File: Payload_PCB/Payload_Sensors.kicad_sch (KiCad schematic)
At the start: 8 parts

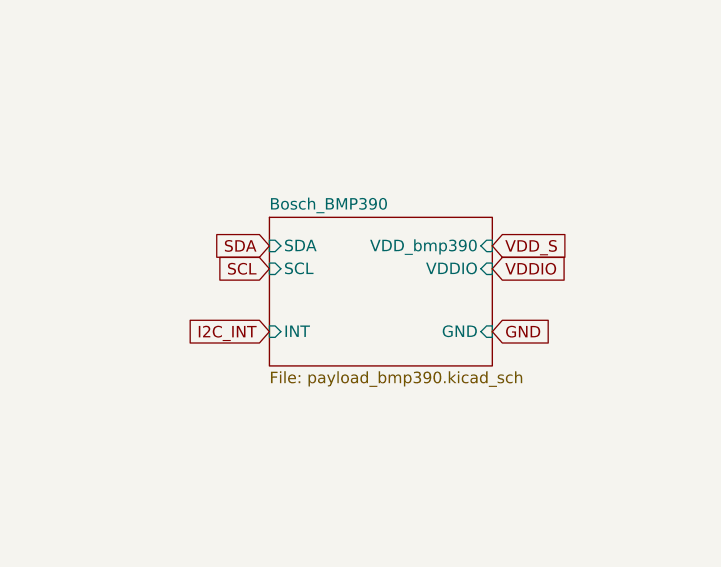
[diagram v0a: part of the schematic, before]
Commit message: some new parts
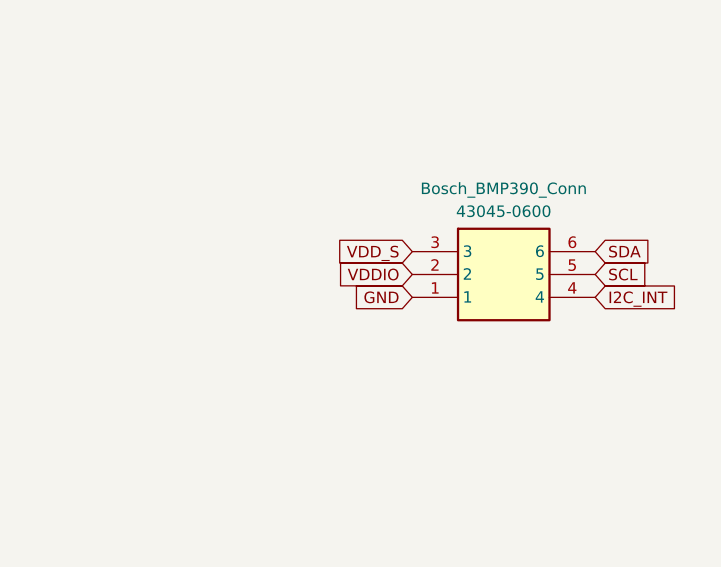
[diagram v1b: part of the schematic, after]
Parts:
- added Bosch_BMP390_Conn: 43045-0600, footprints:43045-06_00,01,02,10_, symbol 43045-0600:43045-0600
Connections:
- net GND: now also Bosch_BMP390_Conn.1
- net I2C_INT: now also Bosch_BMP390_Conn.4
- net SCL: now also Bosch_BMP390_Conn.5
- net SDA: now also Bosch_BMP390_Conn.6
- net VDDIO: now also Bosch_BMP390_Conn.2
- net VDD_S: now also Bosch_BMP390_Conn.3
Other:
- removed sheet Bosch_BMP390
- company: (none) -> SpaceTeam Aachen
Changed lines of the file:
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@@
   (title_block
     (title "Sensor Modules")
+    (company "SpaceTeam Aachen")
   )
   (junction (at 74.295 57.785) (diameter 0) (color 0 0 0 0)
@@
     )
   )
+  (global_label "SCL" (shape input) (at 166.37 210.185 0) (fields_autoplaced)
+    (effects (font (size 1.27 1.27)) (justify left))
+    (property "Intersheetrefs" "${INTERSHEET_REFS}" (at 172.8628 210.185 0)
+      (effects (font (size 1.27 1.27)) (justify left) hide)
+    )
+  )
   (global_label "GND" (shape input) (at 131.445 162.56 0) (fields_autoplaced)
     (effects (font (size 1.27 1.27)) (justify left))
@@
     )
   )
+  (global_label "SDA" (shape input) (at 166.37 207.645 0) (fields_autoplaced)
+    (effects (font (size 1.27 1.27)) (justify left))
+    (property "Intersheetrefs" "${INTERSHEET_REFS}" (at 172.9233 207.645 0)
+      (effects (font (size 1.27 1.27)) (justify left) hide)
+    )
+  )
   (global_label "VDD_TC" (shape input) (at 83.82 43.815 180) (fields_autoplaced)
     (effects (font (size 1.27 1.27)) (justify right))
@@
     )
   )
+  (global_label "GND" (shape input) (at 146.05 212.725 180) (fields_autoplaced)
+    (effects (font (size 1.27 1.27)) (justify right))
+    (property "Intersheetrefs" "${INTERSHEET_REFS}" (at 139.1943 212.725 0)
+      (effects (font (size 1.27 1.27)) (justify right) hide)
+    )
+  )
   (global_label "VDD_TC" (shape input) (at 106.68 151.765 180) (fields_autoplaced)
     (effects (font (size 1.27 1.27)) (justify right))
@@
     )
   )
-  (global_label "VDDIO" (shape input) (at 154.94 209.55 0) (fields_autoplaced)
-    (effects (font (size 1.27 1.27)) (justify left))
-    (property "Intersheetrefs" "${INTERSHEET_REFS}" (at 163.4891 209.55 0)
-      (effects (font (size 1.27 1.27)) (justify left) hide)
-    )
-  )
   (global_label "VDD_TC" (shape input) (at 131.445 74.93 0) (fields_autoplaced)
     (effects (font (size 1.27 1.27)) (justify left))
@@
     )
   )
-  (global_label "SDA" (shape input) (at 130.175 207.01 180) (fields_autoplaced)
-    (effects (font (size 1.27 1.27)) (justify right))
-    (property "Intersheetrefs" "${INTERSHEET_REFS}" (at 123.6217 207.01 0)
-      (effects (font (size 1.27 1.27)) (justify right) hide)
+  (global_label "I2C_INT" (shape input) (at 166.37 212.725 0) (fields_autoplaced)
+    (effects (font (size 1.27 1.27)) (justify left))
+    (property "Intersheetrefs" "${INTERSHEET_REFS}" (at 176.31 212.725 0)
+      (effects (font (size 1.27 1.27)) (justify left) hide)
     )
   )
@@
     )
   )
+  (global_label "VDDIO" (shape input) (at 146.05 210.185 180) (fields_autoplaced)
+    (effects (font (size 1.27 1.27)) (justify right))
+    (property "Intersheetrefs" "${INTERSHEET_REFS}" (at 137.5009 210.185 0)
+      (effects (font (size 1.27 1.27)) (justify right) hide)
+    )
+  )
   (global_label "SCL" (shape input) (at 61.595 55.245 180) (fields_autoplaced)
     (effects (font (size 1.27 1.27)) (justify right))
@@
     )
   )
+  (global_label "VDD_S" (shape input) (at 146.05 207.645 180) (fields_autoplaced)
+    (effects (font (size 1.27 1.27)) (justify right))
+    (property "Intersheetrefs" "${INTERSHEET_REFS}" (at 137.2591 207.645 0)
+      (effects (font (size 1.27 1.27)) (justify right) hide)
+    )
+  )
   (global_label "GND" (shape input) (at 83.82 102.235 180) (fields_autoplaced)
     (effects (font (size 1.27 1.27)) (justify right))
@@
     )
   )
-  (global_label "VDD_S" (shape input) (at 154.94 207.01 0) (fields_autoplaced)
-    (effects (font (size 1.27 1.27)) (justify left))
-    (property "Intersheetrefs" "${INTERSHEET_REFS}" (at 163.7309 207.01 0)
-      (effects (font (size 1.27 1.27)) (justify left) hide)
-    )
-  )
   (global_label "GND" (shape input) (at 131.445 58.42 0) (fields_autoplaced)
     (effects (font (size 1.27 1.27)) (justify left))
@@
     )
   )
-  (global_label "SCL" (shape input) (at 130.175 209.55 180) (fields_autoplaced)
-    (effects (font (size 1.27 1.27)) (justify right))
-    (property "Intersheetrefs" "${INTERSHEET_REFS}" (at 123.6822 209.55 0)
-      (effects (font (size 1.27 1.27)) (justify right) hide)
-    )
-  )
   (global_label "VDD_S" (shape output) (at 66.04 246.38 0) (fields_autoplaced)
     (effects (font (size 1.27 1.27)) (justify left))
@@
     )
   )
-  (global_label "GND" (shape input) (at 154.94 216.535 0) (fields_autoplaced)
-    (effects (font (size 1.27 1.27)) (justify left))
-    (property "Intersheetrefs" "${INTERSHEET_REFS}" (at 161.7957 216.535 0)
-      (effects (font (size 1.27 1.27)) (justify left) hide)
-    )
-  )
   (global_label "VDDIO" (shape output) (at 66.04 264.16 0) (fields_autoplaced)
     (effects (font (size 1.27 1.27)) (justify left))
@@
     (property "Intersheetrefs" "${INTERSHEET_REFS}" (at 75.98 266.7 0)
       (effects (font (size 1.27 1.27)) (justify left) hide)
-    )
-  )
-  (global_label "I2C_INT" (shape input) (at 130.175 216.535 180) (fields_autoplaced)
-    (effects (font (size 1.27 1.27)) (justify right))
-    (property "Intersheetrefs" "${INTERSHEET_REFS}" (at 120.235 216.535 0)
-      (effects (font (size 1.27 1.27)) (justify right) hide)
     )
   )
@@
         (path "/be15da96-a8ba-4b41-94e6-4486ed8c384e"
           (reference "R24") (unit 1)
+        )
+      )
+    )
+  )
+  (symbol (lib_id "43045-0600:43045-0600") (at 146.05 207.645 0) (unit 1)
+    (in_bom yes) (on_board yes) (dnp no) (fields_autoplaced)
+    (property "Reference" "Bosch_BMP390_Conn" (at 156.21 200.66 0)
+      (effects (font (size 1.27 1.27)))
+    )
+    (property "Value" "43045-0600" (at 156.21 203.2 0)
+      (effects (font (size 1.27 1.27)))
+    )
+    (property "Footprint" "footprints:43045-06_00,01,02,10_" (at 162.56 302.565 0)
+      (effects (font (size 1.27 1.27)) (justify left top) hide)
+    )
+    (property "Datasheet" "https://www.molex.com/pdm_docs/sd/430450200_sd.pdf" (at 162.56 402.565 0)
+      (effects (font (size 1.27 1.27)) (justify left top) hide)
+    )
+    (property "Height" "9.9" (at 162.56 602.565 0)
+      (effects (font (size 1.27 1.27)) (justify left top) hide)
+    )
+    (property "Mouser Part Number" "538-43045-0600" (at 162.56 702.565 0)
+      (effects (font (size 1.27 1.27)) (justify left top) hide)
+    )
+    (property "Mouser Price/Stock" "https://www.mouser.co.uk/ProductDetail/Molex/43045-0600?qs=mrPiglD9aYJ8CzJ%2FE2PNbw%3D%3D" (at 162.56 802.565 0)
+      (effects (font (size 1.27 1.27)) (justify left top) hide)
+    )
+    (property "Manufacturer_Name" "Molex" (at 162.56 902.565 0)
+      (effects (font (size 1.27 1.27)) (justify left top) hide)
+    )
+    (property "Manufacturer_Part_Number" "43045-0600" (at 162.56 1002.565 0)
+      (effects (font (size 1.27 1.27)) (justify left top) hide)
+    )
+    (pin "1")
+    (pin "2")
+    (pin "3")
+    (pin "4")
+    (pin "5")
+    (pin "6")
+    (instances
+      (project "Payload_PCB"
+        (path "/5c4f9a68-5778-4223-b18a-2e31db8d7d40/d52ba4fa-6dae-452c-85f1-a72652abf275"
+          (reference "Bosch_BMP390_Conn") (unit 1)
         )
       )
@@
       )
     )
-  )
-  (sheet (at 130.175 203.835) (size 24.765 16.51) (fields_autoplaced)
-    (stroke (width 0.1524) (type solid))
-    (fill (color 0 0 0 0.0000))
-    (property "Sheetname" "Bosch_BMP390" (at 130.175 203.1234 0)
-      (effects (font (size 1.27 1.27)) (justify left bottom))
-    )
-    (property "Sheetfile" "payload_bmp390.kicad_sch" (at 130.175 220.9296 0)
-      (effects (font (size 1.27 1.27)) (justify left top))
-    )
-    (pin "VDDIO" input (at 154.94 209.55 0)
-      (effects (font (size 1.27 1.27)) (justify right))
-    )
-    (pin "SDA" input (at 130.175 207.01 180)
-      (effects (font (size 1.27 1.27)) (justify left))
-    )
-    (pin "INT" input (at 130.175 216.535 180)
-      (effects (font (size 1.27 1.27)) (justify left))
-    )
-    (pin "SCL" input (at 130.175 209.55 180)
-      (effects (font (size 1.27 1.27)) (justify left))
-    )
-    (pin "VDD_bmp390" input (at 154.94 207.01 0)
-      (effects (font (size 1.27 1.27)) (justify right))
-    )
-    (pin "GND" input (at 154.94 216.535 0)
-      (effects (font (size 1.27 1.27)) (justify right))
-    )
-    (instances
-      (project "Payload_PCB"
-        (path "/5c4f9a68-5778-4223-b18a-2e31db8d7d40/d52ba4fa-6dae-452c-85f1-a72652abf275" (page "15"))
-      )
-    )
